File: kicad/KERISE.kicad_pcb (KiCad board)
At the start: 2 copper layers, 42 x 47.5 mm, 116 parts, among them J1 USB_OTG, P1 ANT, P10 Partition, P11 PR_Host, P12 PR_Slave, P13 Partition, P14 Partition, P15 Partition, P16 Partition, P17 COM, P18 Fan, P19 ENC_Host, P2 Motor_L, P20 ENC_Slave, P21 ToF_Host, P22 ToF_Slave, P23 COM, P24 ENC_Host, P25 ENC_Slave, P3 Motor_R, P4 Battery, P5 PR_Host, P6 PR_Slave, P7 Partition, P8 Partition, P9 Partition, Q1 IRFML8244, Q2 IRFML8244, Q3 IRFML8244, Q4 IRFML8244, SW1 SW_Push, SW2 SW_Push, U1 FLASH, U10 MCP73831, U11 FT234XD, U12 AS5048A, U13 ICM-20602, U2 ESP32, U3 XTAL, U4 DRV8835, U5 LXDC2URxx, U6 AD8601, U7 AD8601, U8 AS5048A, U9 VL53L0X

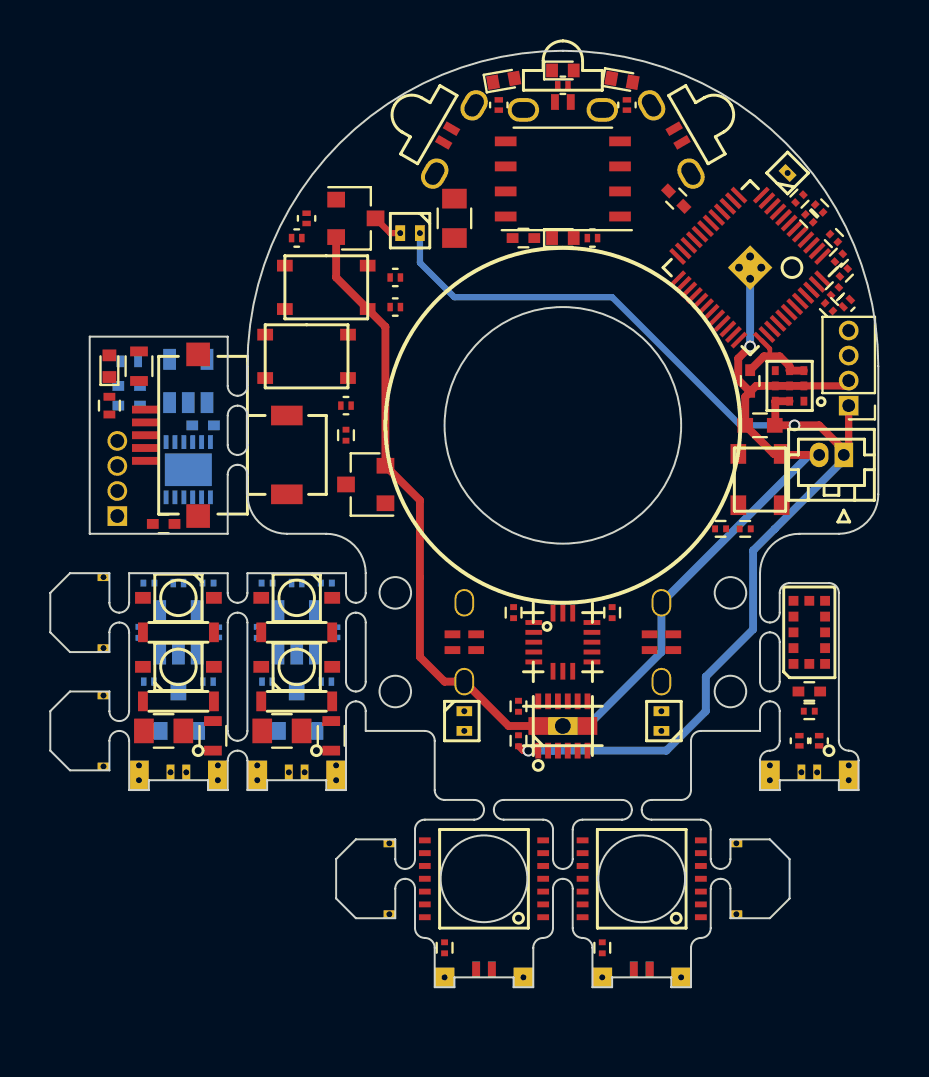
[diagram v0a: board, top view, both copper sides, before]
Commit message: 自動配線成功
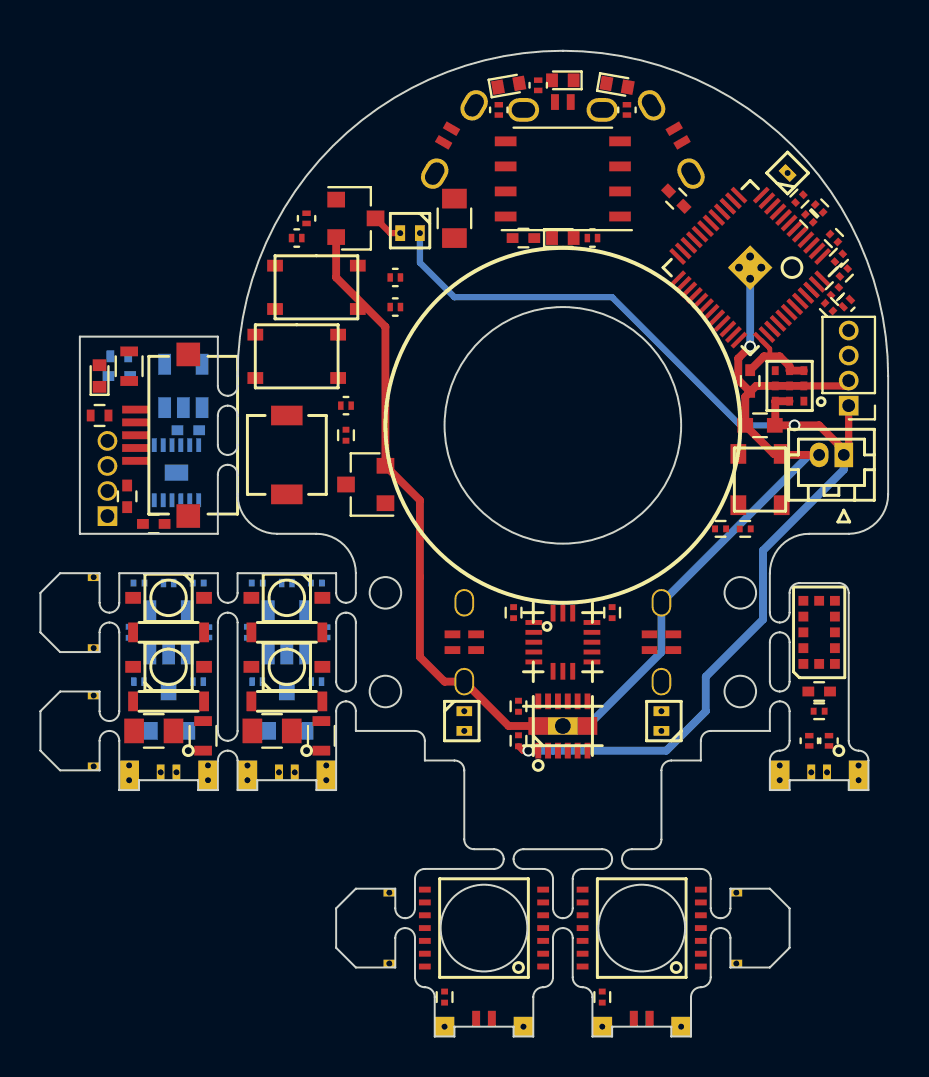
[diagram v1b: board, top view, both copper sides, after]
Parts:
- C32: moved to F.Cu
- U11: footprint Housings_DFN_QFN:DFN-12-1EP_3x3mm_Pitch0.45mm -> mouse:DFN-12-1EP_3x3mm_Pitch0.45mm
- moved C32 4.60 mm to (126.4, 105.6), turned to 90 degrees
- moved C26 2.50 mm to (142.5, 131.0)
- moved C33 2.50 mm to (150.5, 131.0)
- moved P14 2.50 mm to (140.0, 127.5)
- moved P16 2.50 mm to (157.0, 127.5)
- moved P20 2.50 mm to (144.5, 132.5)
- moved P25 2.50 mm to (152.5, 132.5)
- moved U12 2.50 mm to (152.5, 127.5)
- moved U8 2.50 mm to (144.5, 127.5)
- moved R18 1.25 mm to (147.2, 84.8), turned to 90 degrees
- moved C29 0.79 mm to (129.5, 102.2)
- moved C30 0.71 mm to (126.0, 99.5)
- moved D9 0.71 mm to (125.0, 99.5)
- moved R24 0.71 mm to (125.0, 101.5), turned to 0 degrees
- moved U11 0.62 mm to (128.9, 104.4)
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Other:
- board size 42 x 47.5 mm -> 43 x 50 mm
